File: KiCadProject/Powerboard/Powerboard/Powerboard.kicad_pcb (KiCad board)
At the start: 2 copper layers, 45 x 45 mm, 25 parts, among them J1 XT60, J2 XT30, J3 Conn_01x03_Male, Q1 SIR696DP-T1-GE3, Q2 SUD50P10-43L-GE3, U1 MAX16833

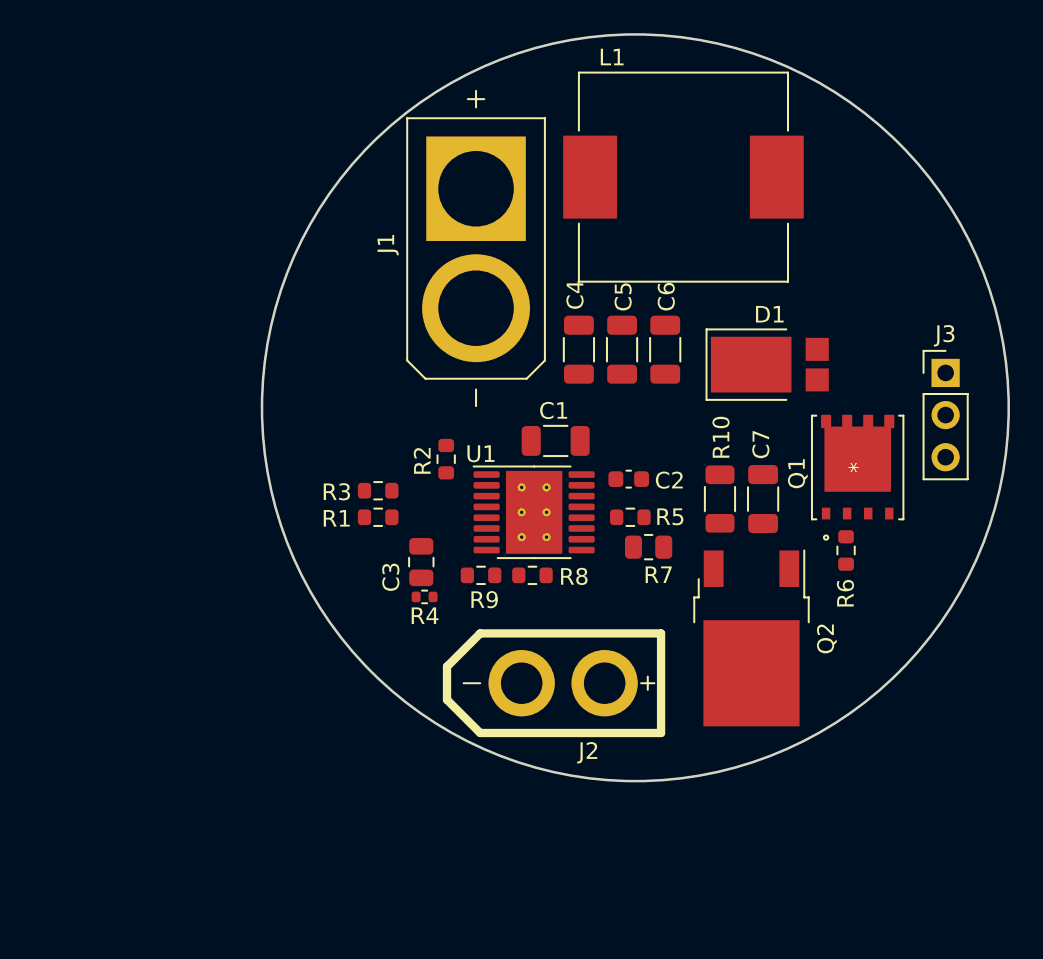
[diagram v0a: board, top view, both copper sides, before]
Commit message: Much more refinement. Re-selected some components for more logical ones. Got all 3d models in place.
Signed-off-by: Eldalote.Electronics <Eldalote.Electronics@gmail.com>
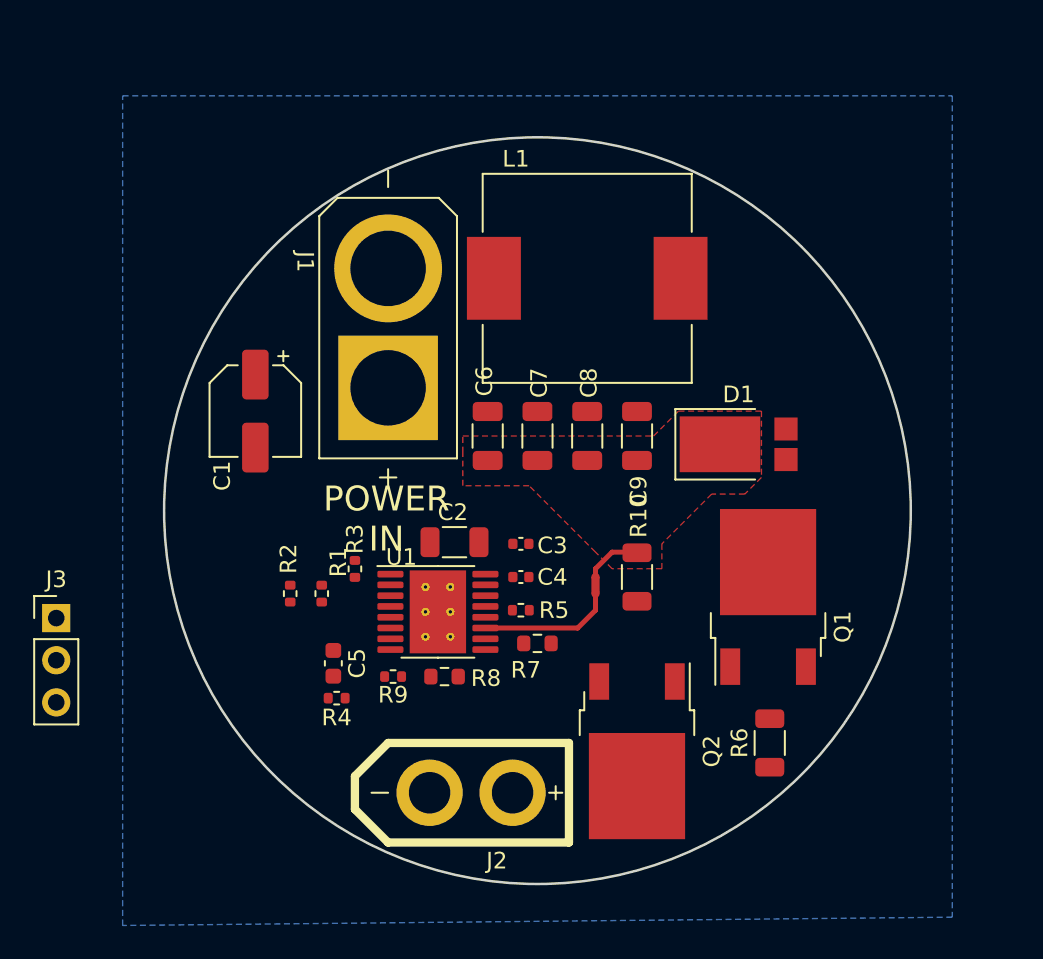
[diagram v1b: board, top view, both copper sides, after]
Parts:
- added C1: Connector cap, Capacitor_SMD:CP_Elec_5x5.3, F.Cu at (133.0, 94.0)
- added C3: 100n, Capacitor_SMD:C_0402_1005Metric, F.Cu at (149.0, 102.0)
- added NT1: NetTie_2, NetTie:NetTie-2_SMD_Pad0.5mm, F.Cu at (153.5, 104.5)
- C4: renamed from C2; footprint Capacitor_SMD:C_0603_1608Metric -> Capacitor_SMD:C_0402_1005Metric
- C5: renamed from C3; value 220n/390n -> 220n; footprint Capacitor_SMD:C_0805_2012Metric -> Capacitor_SMD:C_0603_1608Metric
- L1: value SRP1265C-6R8M -> 6u8
- Q1: value SIR696DP-T1-GE3 -> Q_NMOS_GDS; footprint Ultralibrarianfootprints:SIR696DP-T1-GE3 -> Package_TO_SOT_SMD:TO-252-2
- R1: renamed from R3; footprint Resistor_SMD:R_0603_1608Metric -> Resistor_SMD:R_0402_1005Metric
- R10: value 330m/130m -> 330m
- R2: renamed from R1; footprint Resistor_SMD:R_0603_1608Metric -> Resistor_SMD:R_0402_1005Metric
- R3: renamed from R2; footprint Resistor_SMD:R_0603_1608Metric -> Resistor_SMD:R_0402_1005Metric
- R4: value 953R/120R -> 953R
- R5: value 4k7/2k7 -> 4k7; footprint Resistor_SMD:R_0603_1608Metric -> Resistor_SMD:R_0402_1005Metric
- R6: value 51m/33m -> 51m; footprint Resistor_SMD:R_0603_1608Metric -> Resistor_SMD:R_1206_3216Metric
- R7: footprint Resistor_SMD:R_0805_2012Metric -> Resistor_SMD:R_0603_1608Metric
- R8: value 5M1/4M75 -> 5M1
- R9: footprint Resistor_SMD:R_0603_1608Metric -> Resistor_SMD:R_0402_1005Metric
- moved J3 55.6 mm to (121.0, 106.5)
- moved R6 12.5 mm to (164.0, 114.0)
- moved Q2 9.69 mm to (156.0, 114.5)
- moved Q1 9.49 mm to (163.9, 105.2)
- moved R7 8.86 mm to (150.0, 108.0)
- moved C4 8.78 mm to (149.0, 104.0)
- moved R5 8.66 mm to (149.0, 106.0)
- moved C2 8.63 mm to (145.0, 101.9)
- moved J2 8.62 mm to (146.0, 117.0)
- moved R3 8.60 mm to (139.0, 103.5)
- moved C9 8.50 mm to (156.0, 95.5), turned to 90 degrees
- moved L1 8.42 mm to (153.0, 86.0)
- moved U1 8.35 mm to (144.0, 106.1)
- moved C5 8.08 mm to (137.7, 109.2)
- moved R4 8.08 mm to (137.9, 111.3)
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- renumbered C1 to C2, C4 to C6, C5 to C7, C6 to C8, C7 to C9
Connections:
- net /ISENSE-R renamed /Vout-FET
- C6 pad 1: /ISENSE+ -> /V-out
- C7 pad 1: /ISENSE+ -> /V-out
- C8 pad 1: /ISENSE+ -> /V-out
- C9 pad 1: /ISENSE+ -> /V-out
- D1 pad 1: /ISENSE+ -> /V-out
- D1 pad 2: Net-(D1-Pad2) -> /L-out
- L1 pad 2: Net-(D1-Pad2) -> /L-out
- Q1 pad 1: /RCS -> /NDRV
- Q1 pad 2: /RCS -> /L-out
- R10 pad 2: /ISENSE+ -> /V-out
- R8 pad 2: /ISENSE+ -> /V-out
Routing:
- net /ISENSE+: track 0.00 -> 8.08 mm
- net /V-out: track 0.00 -> 3.43 mm
- added copper zone on F.Cu, net /V-out
- added copper zone on B.Cu, net GND
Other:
- copper layers 2 -> 4
- rule pad_to_mask_clearance: 0 -> 0.05
- board text added: "POWER IN"
